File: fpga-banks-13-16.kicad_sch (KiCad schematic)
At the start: 48 parts, among them U14 XC7A100T-FGG484, U15 Oscillator_100MHz_AMJMEFB

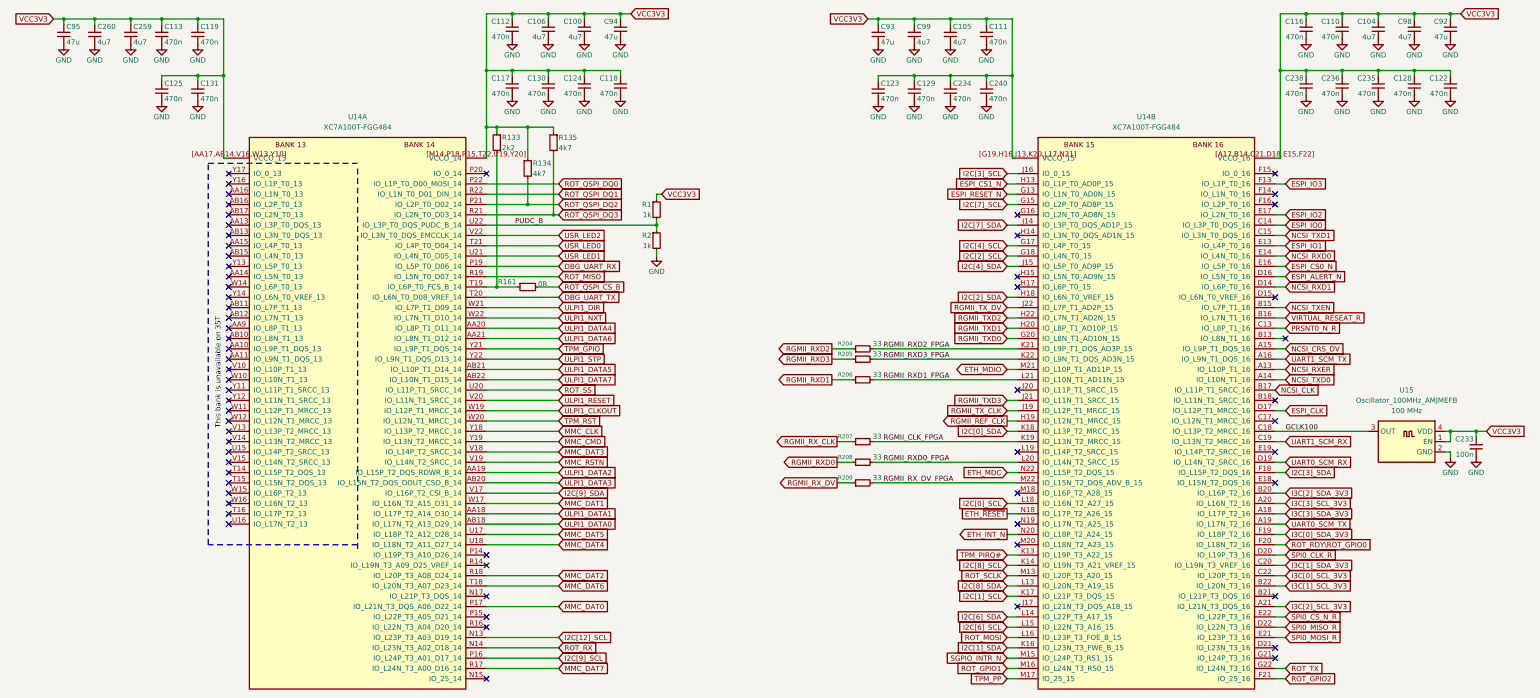
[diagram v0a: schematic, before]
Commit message: pcb final
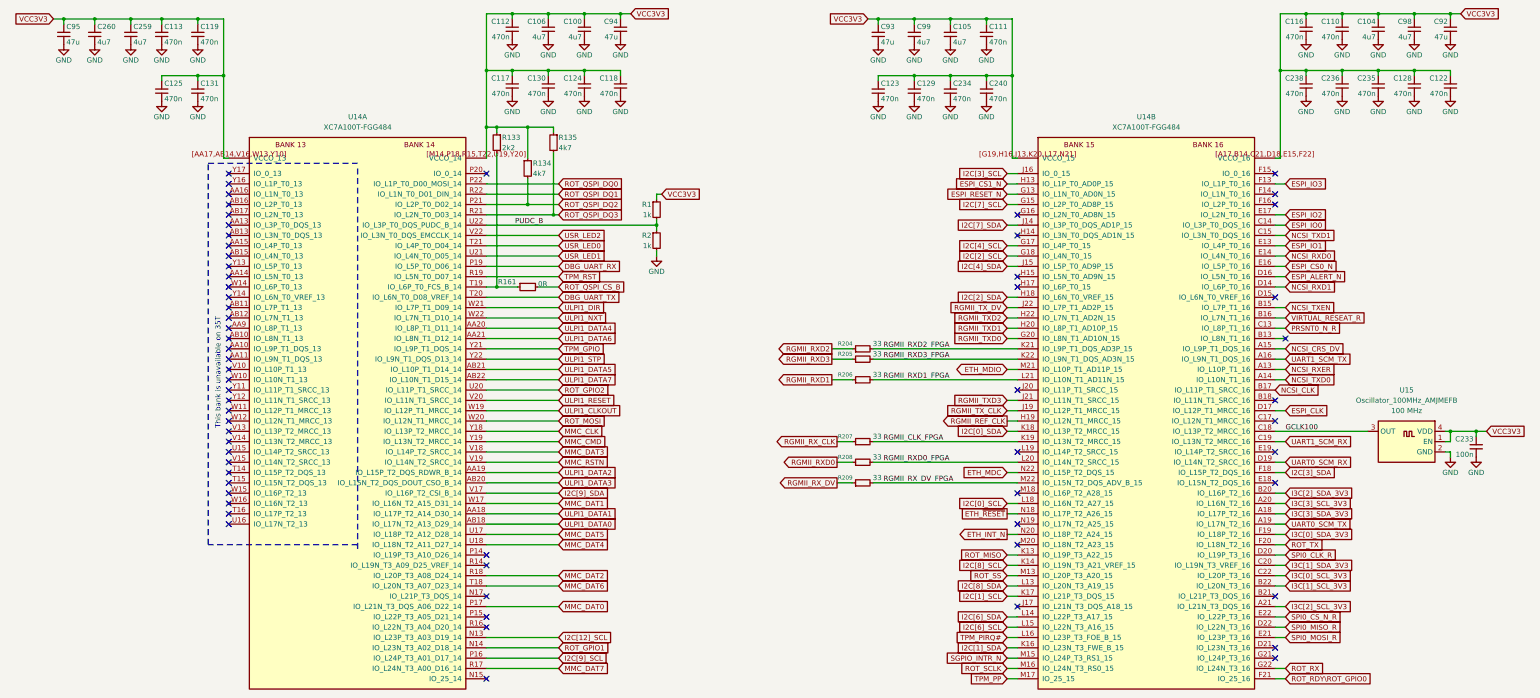
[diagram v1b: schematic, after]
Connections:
- net ROT_GPIO1: now also U14.N14 (IO_L23N_T3_A02_D18_14); no longer U14.M16 (IO_L24N_T3_RS0_15)
- net ROT_GPIO2: now also U14.U20 (IO_L11P_T1_SRCC_14); no longer U14.F21 (IO_25_16)
- net ROT_MISO: now also U14.K13 (IO_L19P_T3_A22_15); no longer U14.R19 (IO_L5N_T0_D07_14)
- net ROT_MOSI: now also U14.W20 (IO_L12N_T1_MRCC_14); no longer U14.L16 (IO_L23P_T3_FOE_B_15)
- net ROT_RDY\ROT_GPIO0: now also U14.F21 (IO_25_16); no longer U14.F20 (IO_L18N_T2_16)
- net ROT_RX: now also U14.G22 (IO_L24N_T3_16); no longer U14.N14 (IO_L23N_T3_A02_D18_14)
- net ROT_SCLK: now also U14.M16 (IO_L24N_T3_RS0_15); no longer U14.M13 (IO_L20P_T3_A20_15)
- net ROT_SS: now also U14.M13 (IO_L20P_T3_A20_15); no longer U14.U20 (IO_L11P_T1_SRCC_14)
- net ROT_TX: now also U14.F20 (IO_L18N_T2_16); no longer U14.G22 (IO_L24N_T3_16)
- net TPM_PIRQ#: now also U14.L16 (IO_L23P_T3_FOE_B_15); no longer U14.K13 (IO_L19P_T3_A22_15)
- net TPM_RST: now also U14.R19 (IO_L5N_T0_D07_14); no longer U14.W20 (IO_L12N_T1_MRCC_14)
